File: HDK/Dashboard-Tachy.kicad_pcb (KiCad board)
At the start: 2 copper layers, 80 x 80 mm, 56 parts, among them J101 Conn_02x08_Odd_Even, U101 CA56-12CGKWA

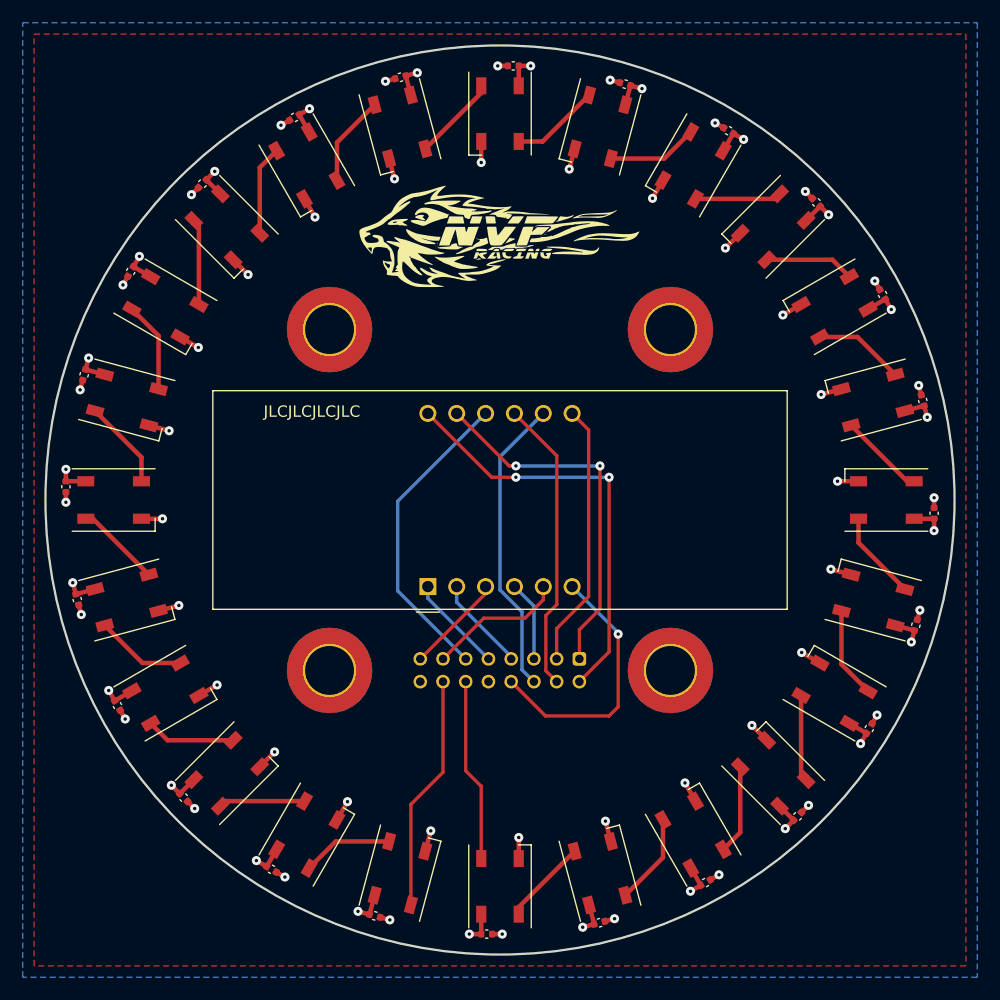
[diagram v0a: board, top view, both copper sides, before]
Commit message: updated REV1.1
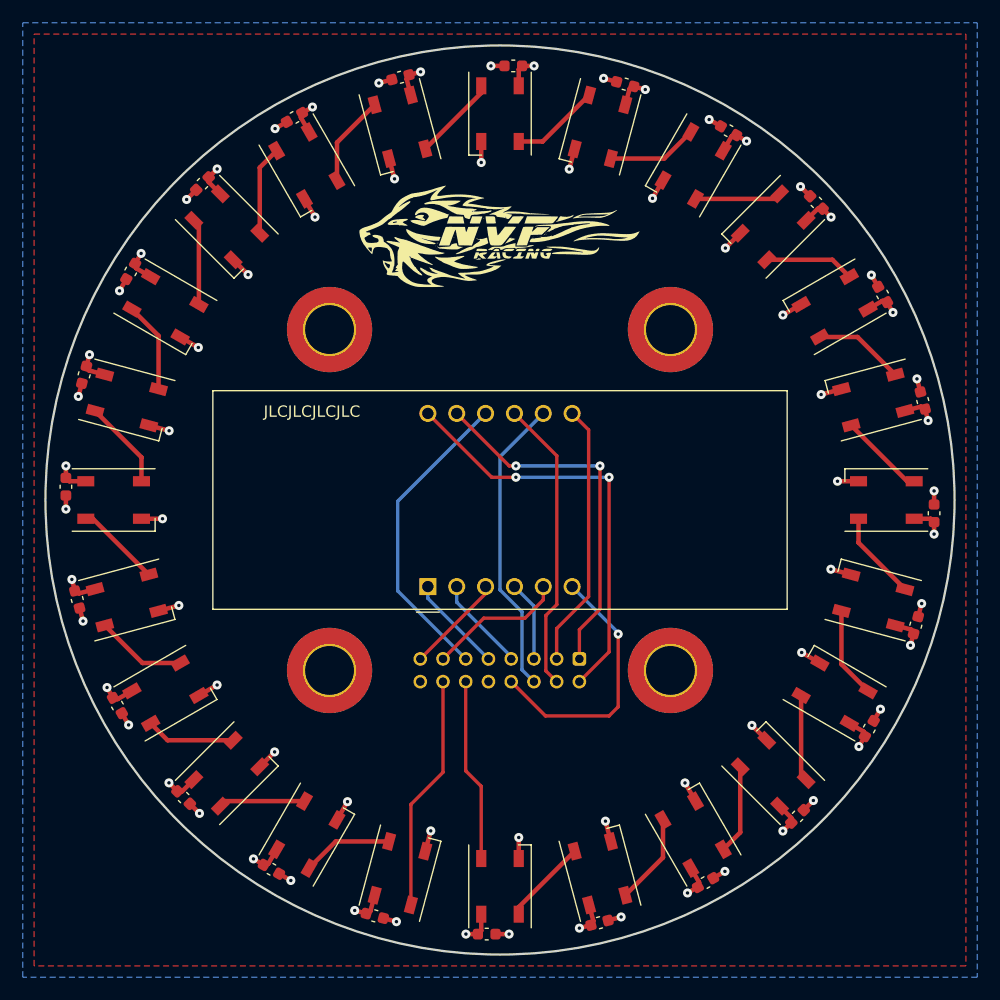
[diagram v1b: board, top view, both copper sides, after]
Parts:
- C101, C102, C103, C104, C105, C106, C107, C108, C109, C110, C111, C112, C113, C114, C115, C116, C117, C118, C119, C120, C121, C122, C123, C124: footprint Capacitor_SMD:C_0402_1005Metric -> Capacitor_SMD:C_0603_1608Metric
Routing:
- net GND: track 65.8 -> 73.1 mm
- net +5V: track 67.2 -> 70.3 mm
